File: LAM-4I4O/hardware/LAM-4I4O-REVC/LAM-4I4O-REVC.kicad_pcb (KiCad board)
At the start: 2 copper layers, 65 x 80 mm, 67 parts, among them J1 MC1,5 2G-3.81, J10 MC 1,5/2G-3,81, J11 MC 1,5/2G-3,81, J12 MC 1,5/2G-3,81, J2 MC1,5 2G-3.81, J3 MC1,5 2G-3.81, J4 PLS, J5 MC 1,5/2G-3,81, J6 MC 1,5/2G-3,81, J7 MC 1,5/2G-3,81, J8 MC 1,5/2G-3,81, J9 MC 1,5/2G-3,81, U1 CH32V003AxMx, U2 SN75176BDR, U3 LT1117-5.0, U4 ULN2003

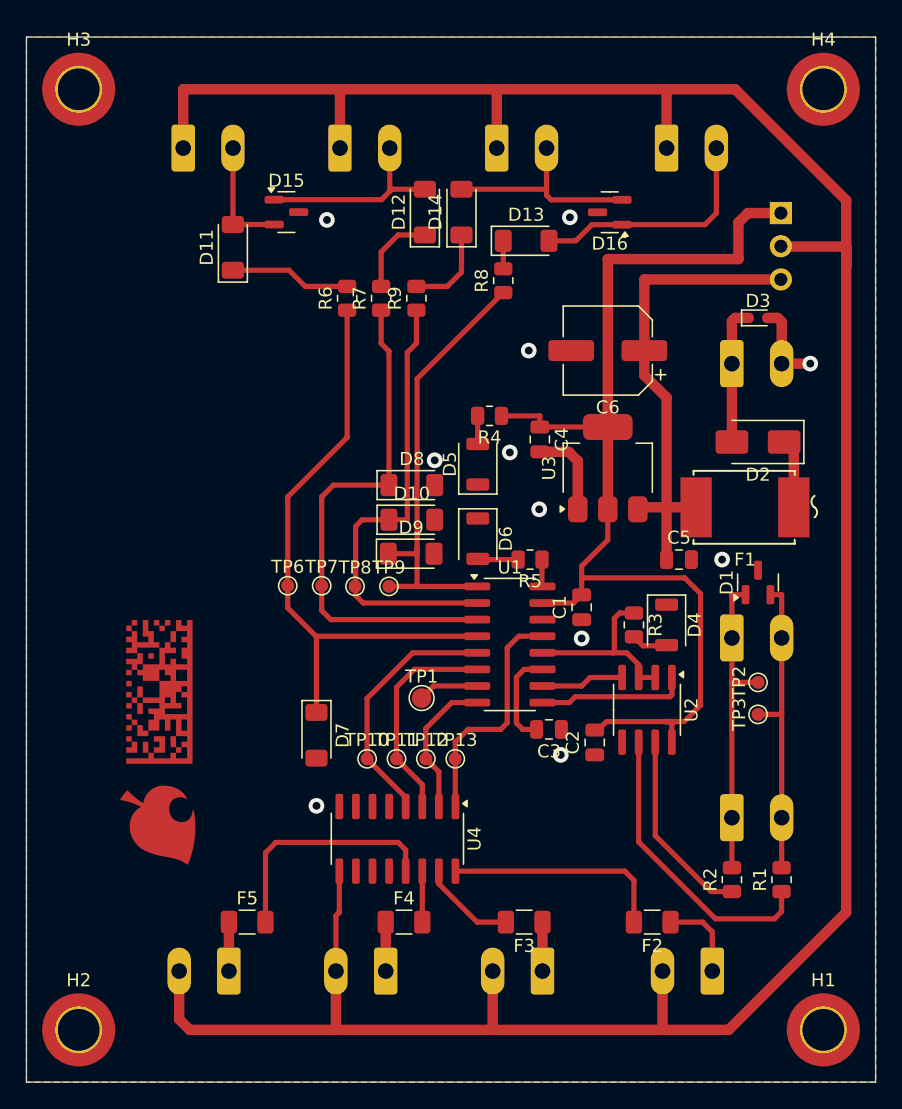
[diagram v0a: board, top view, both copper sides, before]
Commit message: fix(LAM-4I4O): increase trace length to 0.5mm, fix missing ground trace for single-layer manufacturing
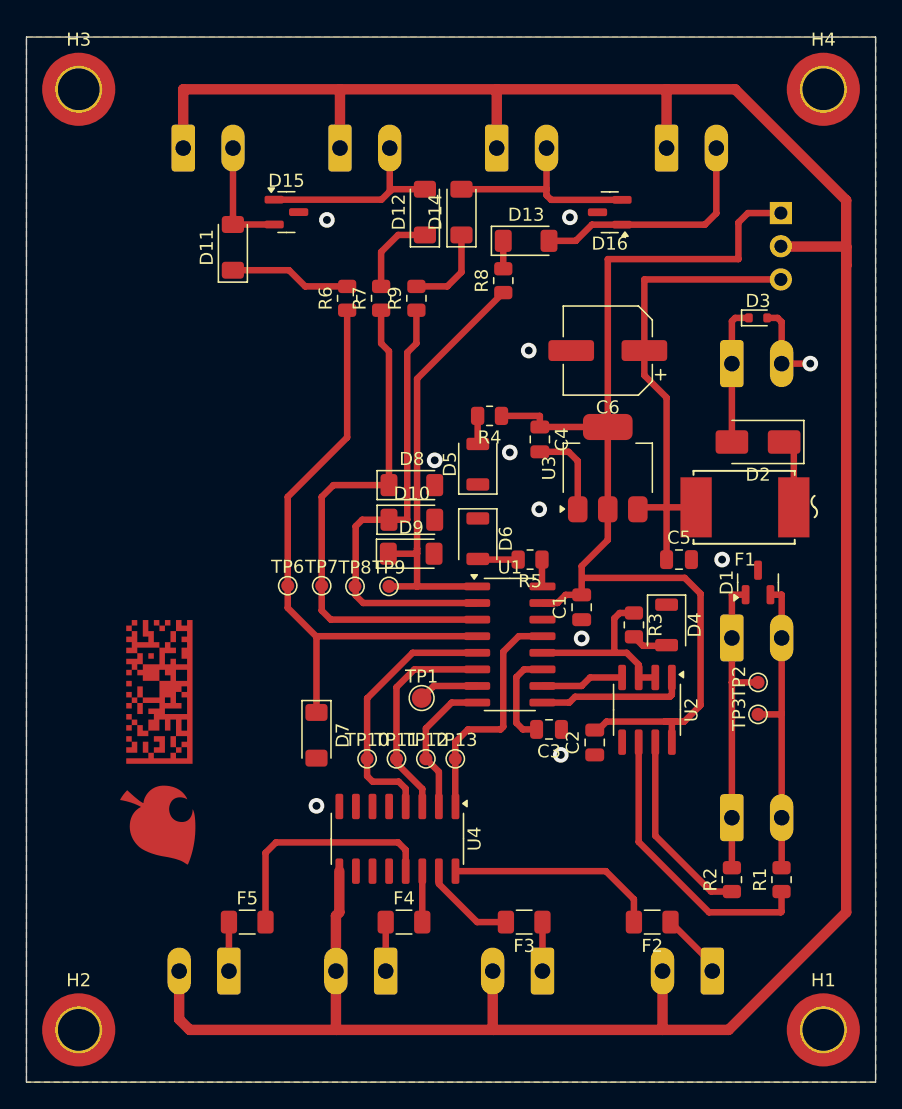
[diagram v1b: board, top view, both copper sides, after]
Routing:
- net Net-(J9-Pin_1): track 6.51 -> 5.08 mm
- net /OUT1: track 18.7 -> 19.8 mm
- net Net-(U4-O1): track 17.1 -> 16.3 mm
